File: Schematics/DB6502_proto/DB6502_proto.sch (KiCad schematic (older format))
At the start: 23 parts, among them U1 71256, U2 71256, U3 28C256, U4 65C02S, U5 74AC74, U6 74AC138, U7 22V10C, U8 74AC04, U9 74HC21

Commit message: Working on a PCB
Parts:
- RN1: footprint Resistor_THT:R_Array_SIP5 -> Resistor_THT:R_Array_SIP9; symbol Device:R_Network04 -> Device:R_Network08
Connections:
- net BE: now also RN1.9 (R8)
- net ~NMI: now also RN1.8 (R7)
- net ~SO: now also RN1.7 (R6)
- new net SR_OUT: RN1.6 (R5)
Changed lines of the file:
@@
 Wire Wire Line
 	5100 7450 5650 7450
-Text GLabel 4450 6550 1    50   Input ~ 0
+Text GLabel 3800 5950 1    50   Input ~ 0
 +5V
 Text GLabel 2850 7150 0    50   Input ~ 0
@@
 PLD_CLK
 $Comp
-L Device:R_Network04 RN1
+L Device:R_Network08 RN1
 U 1 1 6054D542
-P 4650 6850
-F 0 "RN1" H 4838 6896 50  0000 L CNN
-F 1 "4K7" H 4838 6805 50  0000 L CNN
-F 2 "Resistor_THT:R_Array_SIP5" V 4925 6850 50  0001 C CNN
-F 3 "http://www.vishay.com/docs/31509/csc.pdf" H 4650 6850 50  0001 C CNN
-	1    4650 6850
-	1    0    0    -1
-$EndComp
-Wire Wire Line
-	4450 6550 4450 6650
-Wire Wire Line
-	4750 7050 4750 7150
-Wire Wire Line
-	4750 7150 5550 7150
+P 4200 6250
+F 0 "RN1" H 4600 6300 50  0000 L CNN
+F 1 "4K7" H 4600 6200 50  0000 L CNN
+F 2 "Resistor_THT:R_Array_SIP9" V 4475 6250 50  0001 C CNN
+F 3 "http://www.vishay.com/docs/31509/csc.pdf" H 4200 6250 50  0001 C CNN
+	1    4200 6250
+	1    0    0    -1
+$EndComp
+Wire Wire Line
+	3800 5950 3800 6050
+Wire Wire Line
+	4100 6450 4100 7150
+Wire Wire Line
+	4100 7150 5550 7150
 Connection ~ 5550 7150
 Wire Wire Line
-	4650 7050 4650 7250
-Wire Wire Line
-	4650 7250 5400 7250
+	4000 6450 4000 7250
+Wire Wire Line
+	4000 7250 5400 7250
 Connection ~ 5400 7250
 Wire Wire Line
-	4550 7050 4550 7350
-Wire Wire Line
-	4550 7350 5250 7350
+	3900 6450 3900 7350
+Wire Wire Line
+	3900 7350 5250 7350
 Connection ~ 5250 7350
 Wire Wire Line
-	4450 7050 4450 7450
-Wire Wire Line
-	4450 7450 5100 7450
+	3800 6450 3800 7450
+Wire Wire Line
+	3800 7450 5100 7450
 Connection ~ 5100 7450
+Text GLabel 4600 6550 2    50   Output ~ 0
+BE
+Wire Wire Line
+	4500 6550 4500 6450
+Text GLabel 4600 6700 2    50   Output ~ 0
+~NMI
+Wire Wire Line
+	4500 6550 4600 6550
+Wire Wire Line
+	4600 6700 4400 6700
+Wire Wire Line
+	4400 6700 4400 6450
+Text GLabel 4600 6850 2    50   Output ~ 0
+~SO
+Wire Wire Line
+	4300 6450 4300 6850
+Wire Wire Line
+	4300 6850 4600 6850
+Text GLabel 4600 7000 2    50   Output ~ 0
+SR_OUT
+Wire Wire Line
+	4600 7000 4200 7000
+Wire Wire Line
+	4200 7000 4200 6450
 Wire Bus Line
 	8500 4150 8500 4350

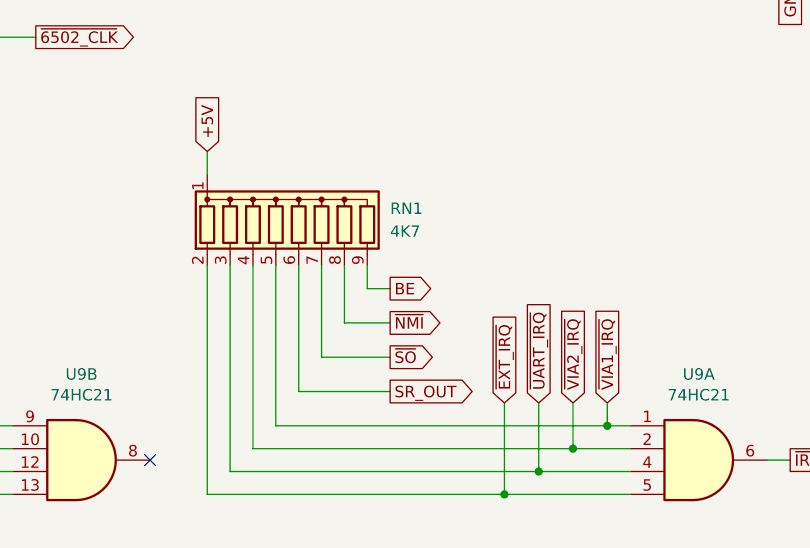
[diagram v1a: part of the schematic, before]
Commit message: Small fixes on PCB
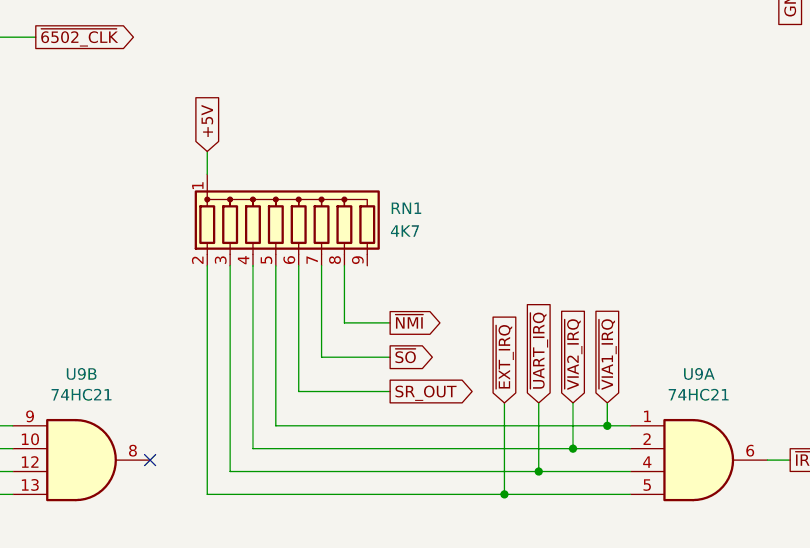
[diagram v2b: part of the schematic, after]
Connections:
- net BE: no longer RN1.9 (R8)
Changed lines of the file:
@@
 	3800 7450 5100 7450
 Connection ~ 5100 7450
-Text GLabel 4600 6550 2    50   Output ~ 0
-BE
-Wire Wire Line
-	4500 6550 4500 6450
 Text GLabel 4600 6700 2    50   Output ~ 0
 ~NMI
 Wire Wire Line
-	4500 6550 4600 6550
-Wire Wire Line
 	4600 6700 4400 6700
